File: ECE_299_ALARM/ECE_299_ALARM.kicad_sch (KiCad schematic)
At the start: 16 parts, among them SW1 SW_Push_Dual, SW2 SW_Push_Dual, SW3 SW_Push_Dual, SW4 SW_Push_Dual, U1 RDA5807M_Module, U2 RPi_Pico_TH, U3 LM386

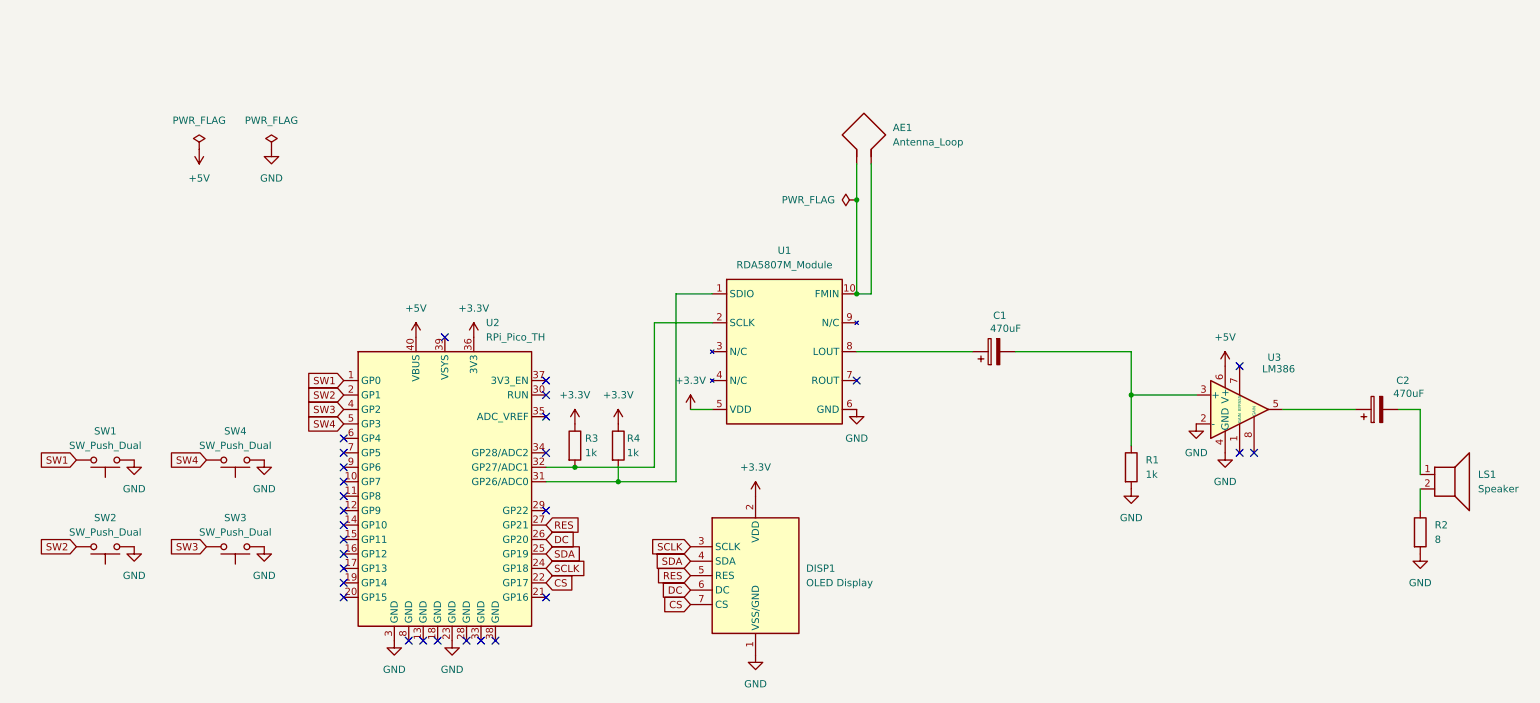
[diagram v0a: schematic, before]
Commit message: small_adjustments
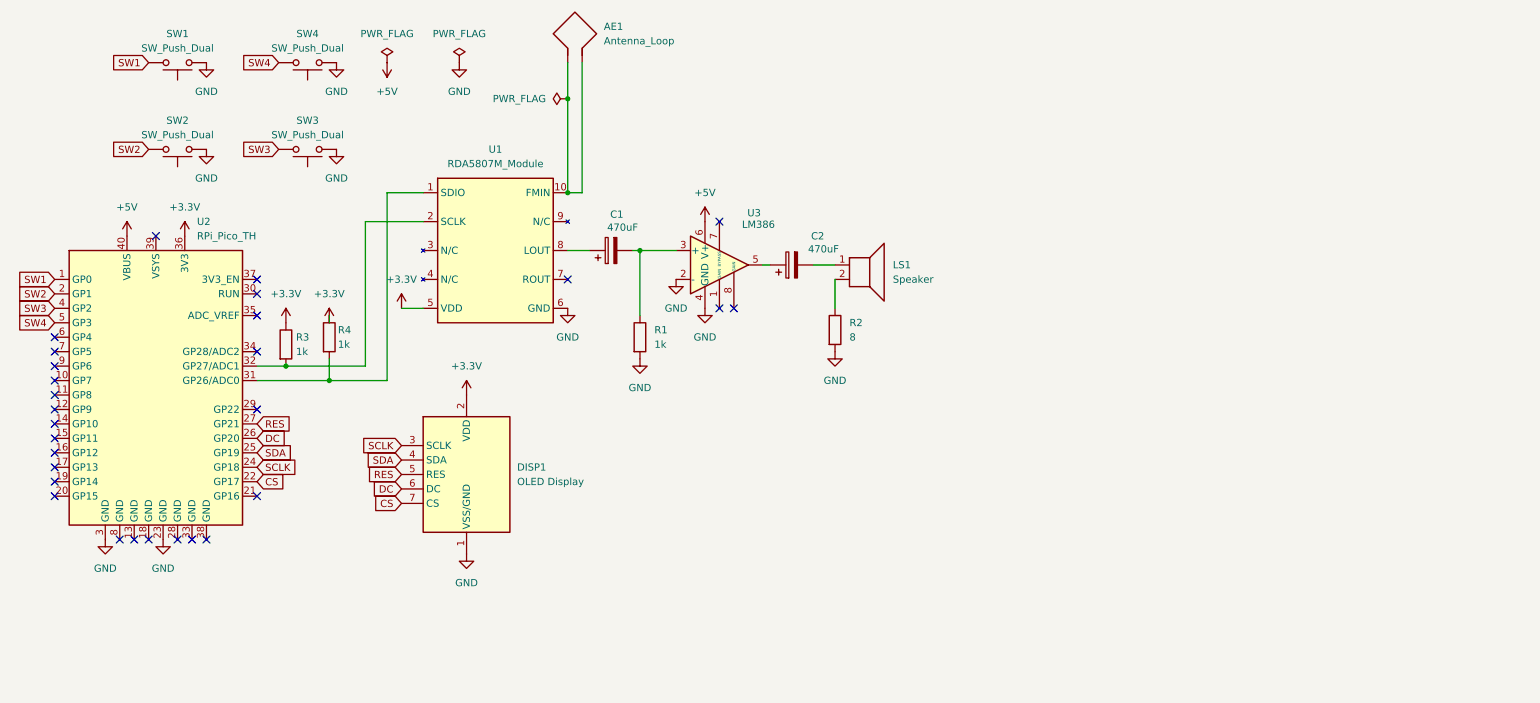
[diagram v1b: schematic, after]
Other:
- moved on the sheet: AE1, C1, C2, DISP1, LS1, R1, R2, R3, R4, SW1, SW2, SW3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
